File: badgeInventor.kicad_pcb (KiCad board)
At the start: 2 copper layers, 89.2 x 86 mm, 35 parts, among them P1 AUTO-PROGRAM JUMPER, P2 CONN_01X10, P22 CONN_01X10, P23 CONN_01X10, P3 LiPo, P5 OLED_I2C, P6 USB Serial, SW1 RESET, U1 SPX1117, U2 MCP73831, U3 ESP-12E

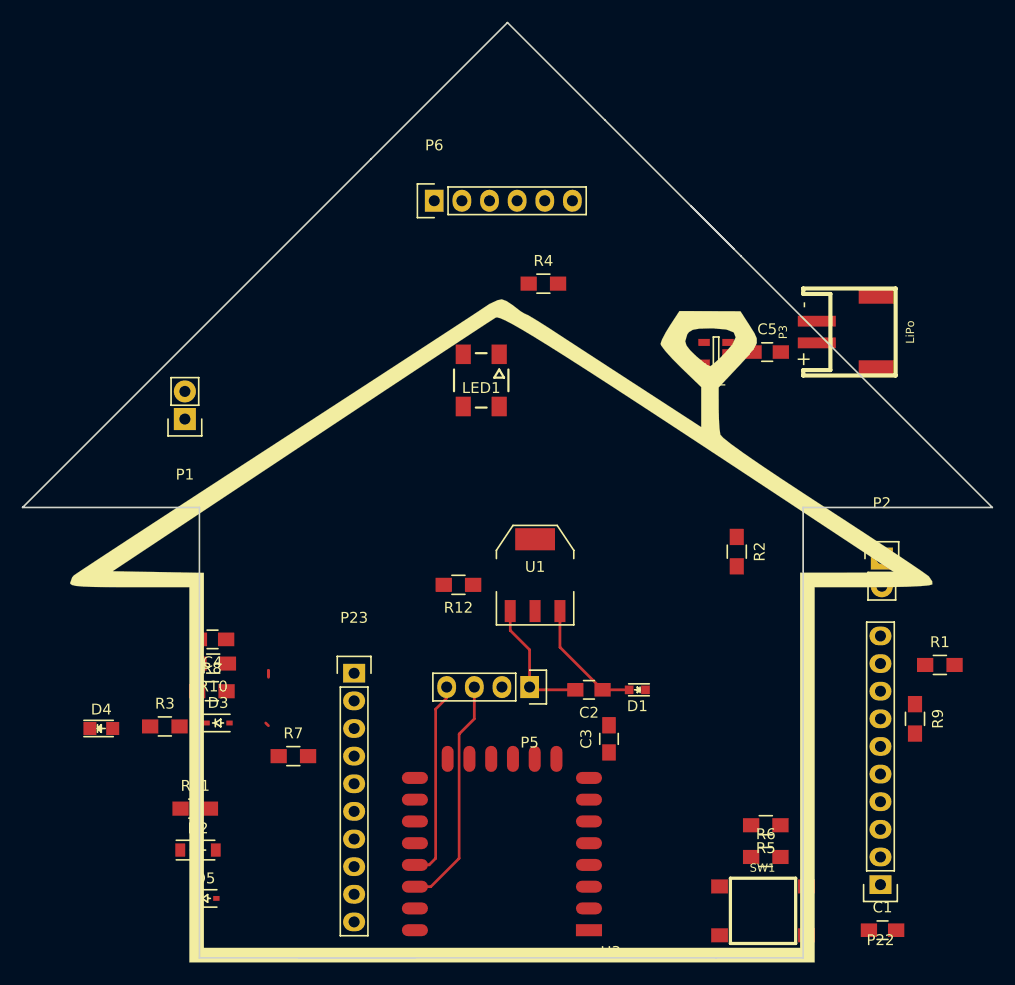
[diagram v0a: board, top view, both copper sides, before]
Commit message: PCB v0.01
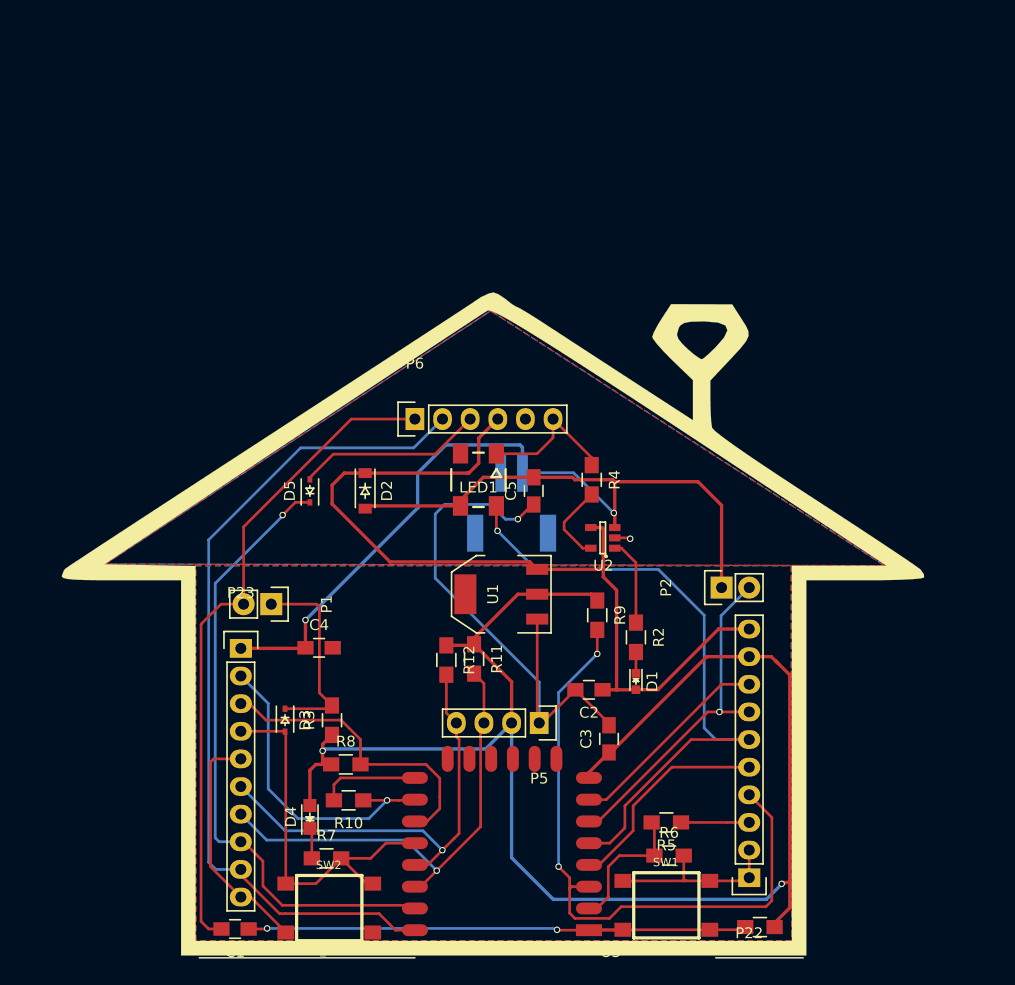
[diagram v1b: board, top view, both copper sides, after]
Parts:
- added SW2: SW_PUSH, open-project:SW_PUSH_SMD, F.Cu at (124.5, 146.3)
- P3: moved to B.Cu
- moved C1 59.5 mm to (115.8, 148.2), turned to 180 degrees
- moved P3 40.7 mm to (141.2, 113.5), turned to 180 degrees
- moved D5 38.7 mm to (122.7, 108.0), turned to 90 degrees
- moved D2 36.4 mm to (127.8, 108.0), turned to 270 degrees
- moved R9 30.7 mm to (149.1, 119.4)
- moved R1 29.2 mm to (164.1, 148.1), turned to 180 degrees
- moved R11 29.1 mm to (137.8, 123.4), turned to 270 degrees
- moved C5 25.0 mm to (143.3, 108.0), turned to 90 degrees
- moved D4 20.8 mm to (122.7, 137.9), turned to 90 degrees
- moved P6 20.1 mm to (132.3, 101.3)
- moved U2 20.0 mm to (149.6, 112.3)
- moved P1 18.8 mm to (119.1, 118.4), turned to 270 degrees
- moved R4 18.6 mm to (148.6, 106.9), turned to 270 degrees
- moved R10 17.7 mm to (126.2, 136.4)
- moved R3 15.4 mm to (124.7, 129.0), turned to 90 degrees
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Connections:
- P22 pad 2: /ESP8266/GPIO0 -> GND
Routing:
- net +3V3: track 1.24 -> 142.5 mm, vias 0 -> 2
- net GND: track 12.6 -> 115.2 mm, vias 0 -> 2
- net +BATT: track 0.00 -> 98.6 mm, vias 0 -> 2
- net /ESP8266/RX: track 0.00 -> 77.6 mm
- net VCC: track 11.3 -> 80.6 mm
- net /ESP8266/DTR: track 0.00 -> 61.9 mm
- net /ESP8266/GPIO14: track 0.00 -> 60.3 mm, vias 0 -> 1
- net /ESP8266/CH_PD: track 0.00 -> 59.9 mm, vias 0 -> 2
- net /ESP8266/TX: track 0.05 -> 57.7 mm, vias 0 -> 1
- net /ESP8266/RST: track 0.66 -> 49.4 mm, vias 0 -> 2
- net /ESP8266/GPIO0: track 0.12 -> 35.4 mm
- net /ESP8266/GPIO12: track 0.00 -> 31.5 mm, vias 0 -> 1
- net /ESP8266/GPIO15: track 0.00 -> 28.9 mm, vias 0 -> 1
- net /ESP8266/GPIO2: track 0.23 -> 28.3 mm
- net /ESP8266/GPIO4/SDA: track 18.3 -> 41.3 mm, vias 0 -> 1
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- added copper zone on B.Cu, net GND
- added copper zone on F.Cu, net GND
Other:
- board outline removed
- net class Vcc added: clearance 0.2, trace_width 0.31, via_dia 0.6, via_drill 0.4
